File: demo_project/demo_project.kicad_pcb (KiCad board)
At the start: 2 copper layers, 105 x 80 mm, 22 parts, among them Q101 2N7000, SW101 LEFT, SW102 UP, SW103 RIGHT, SW104 DOWN

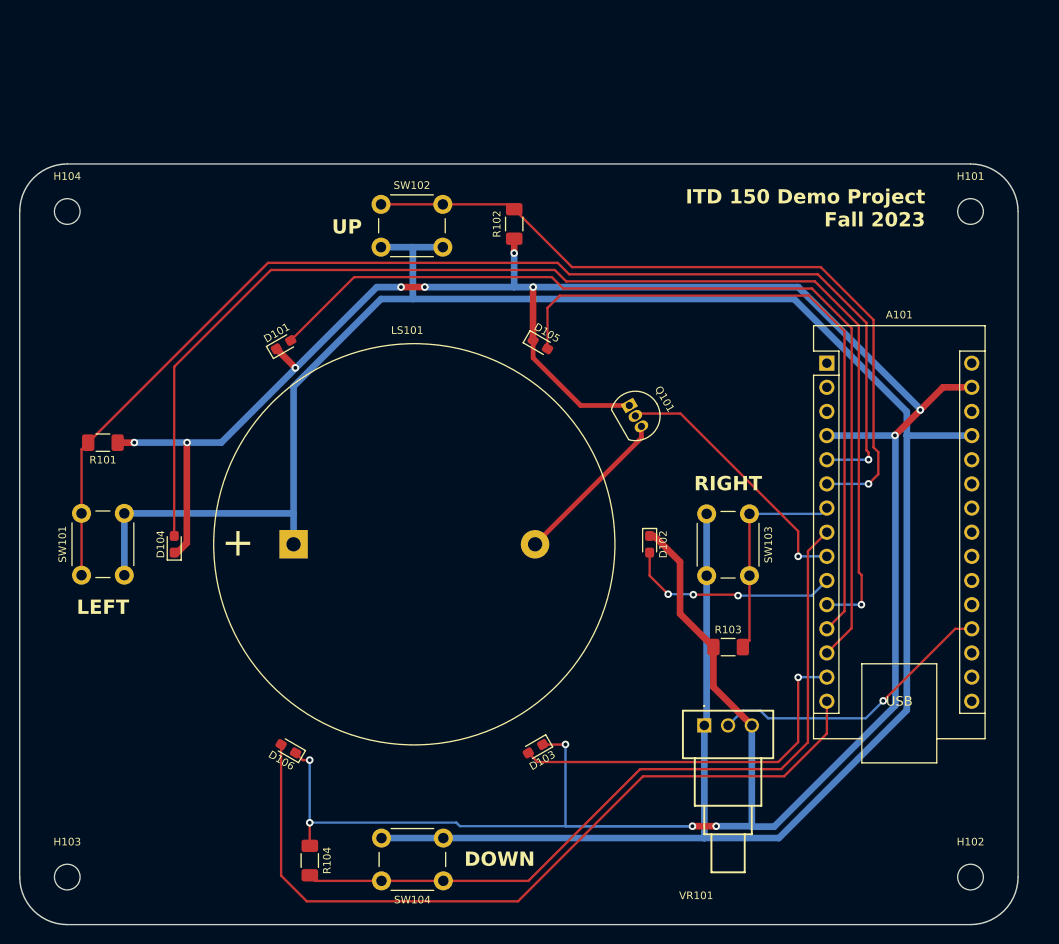
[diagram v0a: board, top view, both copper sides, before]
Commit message: blank sch starter
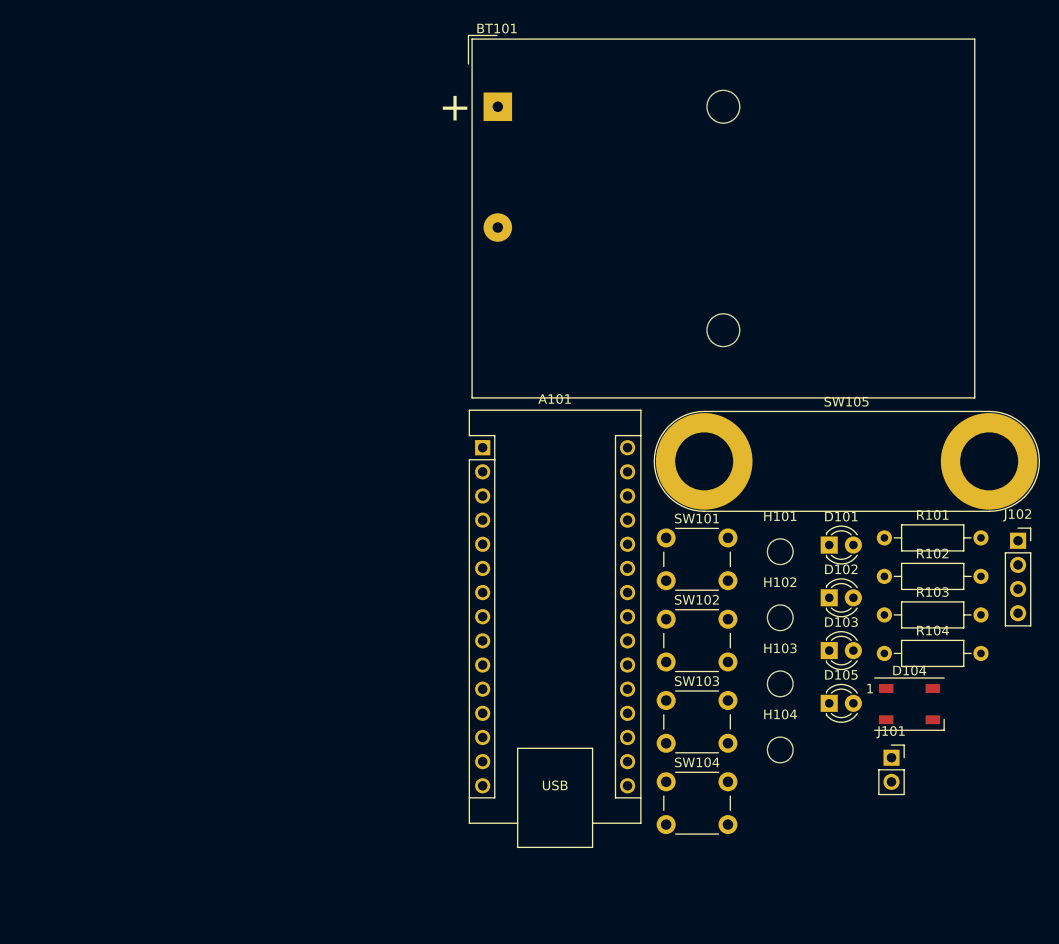
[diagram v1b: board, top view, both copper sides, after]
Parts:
- removed D106: BLUE, LED_SMD:LED_0603_1608Metric_Pad1.05x0.95mm_HandSolder
- removed LS101: Speaker, Buzzer_Beeper:MagneticBuzzer_ProjectsUnlimited_AI-4228-TWT-R
- removed Q101: 2N7000, Package_TO_SOT_THT:TO-92_Inline
- removed VR101: RK09Y11L0001, footprints:alps_alpine_RK09Y11L0001
- added BT101: Battery, Battery:BatteryHolder_Keystone_2479_3xAAA, F.Cu at (125.3, 54.0)
- added J101: Conn_01x02, Connector_PinSocket_2.54mm:PinSocket_1x02_P2.54mm_Vertical, F.Cu at (166.7, 122.5)
- added J102: Conn_01x04, Connector_PinSocket_2.54mm:PinSocket_1x04_P2.54mm_Vertical, F.Cu at (180.0, 99.6)
- added SW105: SW_SPST, Connector:Banana_Jack_2Pin, F.Cu at (147.0, 91.3)
- D101: footprint LED_SMD:LED_0603_1608Metric_Pad1.05x0.95mm_HandSolder -> LED_THT:LED_D3.0mm_FlatTop
- D102: value YELLOW -> GREEN; footprint LED_SMD:LED_0603_1608Metric_Pad1.05x0.95mm_HandSolder -> LED_THT:LED_D3.0mm_FlatTop
- D103: value GREEN -> BLUE; footprint LED_SMD:LED_0603_1608Metric_Pad1.05x0.95mm_HandSolder -> LED_THT:LED_D3.0mm_FlatTop
- D104: value GREEN -> WS2812B; footprint LED_SMD:LED_0603_1608Metric_Pad1.05x0.95mm_HandSolder -> LED_SMD:LED_WS2812B_PLCC4_5.0x5.0mm_P3.2mm
- D105: value BLUE -> GREEN; footprint LED_SMD:LED_0603_1608Metric_Pad1.05x0.95mm_HandSolder -> LED_THT:LED_D3.0mm_FlatTop
- R101, R102, R103, R104: footprint Resistor_SMD:R_1206_3216Metric_Pad1.30x1.75mm_HandSolder -> Resistor_THT:R_Axial_DIN0207_L6.3mm_D2.5mm_P10.16mm_Horizontal
- moved H104 94.0 mm to (155.0, 121.6)
- moved R101 82.8 mm to (165.9, 99.3), turned to 0 degrees
- moved D104 79.1 mm to (168.6, 116.8), turned to 0 degrees
- moved H103 77.7 mm to (155.0, 114.7)
- moved R104 64.2 mm to (165.9, 111.5), turned to 0 degrees
- moved SW101 61.6 mm to (143.0, 99.3), turned to 0 degrees
- moved D101 61.1 mm to (160.1, 100.1), turned to 0 degrees
- moved R102 53.8 mm to (165.9, 103.4), turned to 0 degrees
- moved SW102 52.9 mm to (143.0, 107.9)
- moved D105 48.4 mm to (160.1, 116.7), turned to 0 degrees
- moved H101 41.0 mm to (155.0, 100.8)
- moved A101 37.3 mm to (123.7, 89.8)
- moved H102 33.8 mm to (155.0, 107.7)
- moved D103 32.6 mm to (160.1, 111.2), turned to 0 degrees
- moved SW104 25.7 mm to (143.0, 125.0), turned to 0 degrees
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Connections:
- A101 pad 10: /LED_YELLOW -> unconnected-(A101-D7-Pad10)
- A101 pad 11: /LED_GREEN -> unconnected-(A101-D8-Pad11)
- A101 pad 12: /LED_BLUE_PWM -> unconnected-(A101-D9-Pad12)
- A101 pad 13: /LED_YELLOW_PWM -> unconnected-(A101-D10-Pad13)
- A101 pad 14: /LED_GREEN_PWM -> unconnected-(A101-D11-Pad14)
- A101 pad 15: /LED_BLUE -> unconnected-(A101-D12-Pad15)
- A101 pad 19: /POTENTIOMETER_AIN -> unconnected-(A101-A0-Pad19)
- A101 pad 30: unconnected-(A101-VIN-Pad30) -> /VIN
- A101 pad 9: /SPEAKER_PWM -> unconnected-(A101-D6-Pad9)
- D101 pad 1: GND -> unconnected-(D101-K-Pad1)
- D101 pad 2: /LED_YELLOW_PWM -> unconnected-(D101-A-Pad2)
- D102 pad 1: GND -> unconnected-(D102-K-Pad1)
- D102 pad 2: /LED_YELLOW -> unconnected-(D102-A-Pad2)
- D103 pad 1: GND -> unconnected-(D103-K-Pad1)
- D103 pad 2: /LED_GREEN_PWM -> unconnected-(D103-A-Pad2)
- D104 pad 1: GND -> unconnected-(D104-VDD-Pad1)
- D104 pad 2: /LED_GREEN -> unconnected-(D104-DOUT-Pad2)
- D105 pad 1: GND -> unconnected-(D105-K-Pad1)
- D105 pad 2: /LED_BLUE_PWM -> unconnected-(D105-A-Pad2)
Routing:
- net GND: track 319.8 -> 0.00 mm, vias 14 -> 0
- net +5V: track 259.3 -> 0.00 mm
- net /LED_GREEN: track 129.6 -> 0.00 mm, vias 1 -> 0
- net /LEFT: track 125.3 -> 0.00 mm, vias 1 -> 0
- net /LED_YELLOW_PWM: track 99.2 -> 0.00 mm
- net /LED_BLUE: track 83.0 -> 0.00 mm
- net /DOWN: track 81.6 -> 0.00 mm
- net /UP: track 79.1 -> 0.00 mm, vias 1 -> 0
- net /LED_BLUE_PWM: track 69.7 -> 0.00 mm
- net /LED_GREEN_PWM: track 39.4 -> 0.00 mm, vias 1 -> 0
- net /POTENTIOMETER_AIN: track 30.5 -> 0.00 mm, vias 1 -> 0
- net /SPEAKER_PWM: track 28.0 -> 0.00 mm, vias 1 -> 0
- net /RIGHT: track 22.7 -> 0.00 mm
- net /LED_YELLOW: track 22.6 -> 0.00 mm, vias 3 -> 0
- net Net-(Q101-D): track 17.0 -> 0.00 mm
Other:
- board outline removed
- board text removed: "DOWN"
- board text removed: "ITD 150 Demo Project Fall 2023"
- board text removed: "LEFT"
- board text removed: "RIGHT"
- board text removed: "UP"
